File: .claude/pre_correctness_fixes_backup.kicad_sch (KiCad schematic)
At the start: 64 parts, among them J1 USB_C_Receptacle_USB2.0_16P, J10 5055670271, J12 5054482071, J2 5055670271, J3 SM04B-GHS-TB, J4 XT30 (right-angle), J5 SM04B-GHS-TB, J6 5055670271, J7 5055670271, J8 5055670271, Q1 DMP3098L-7, SW1 B3U-1000P, SW2 B3U-1000P, U1 USBLC6-2SC6, U2 AMS1117-3.3, U3 ESP32-S3-WROOM-1, U4 TJA1051T/3, U5 AP3602A, U6 LMR33630

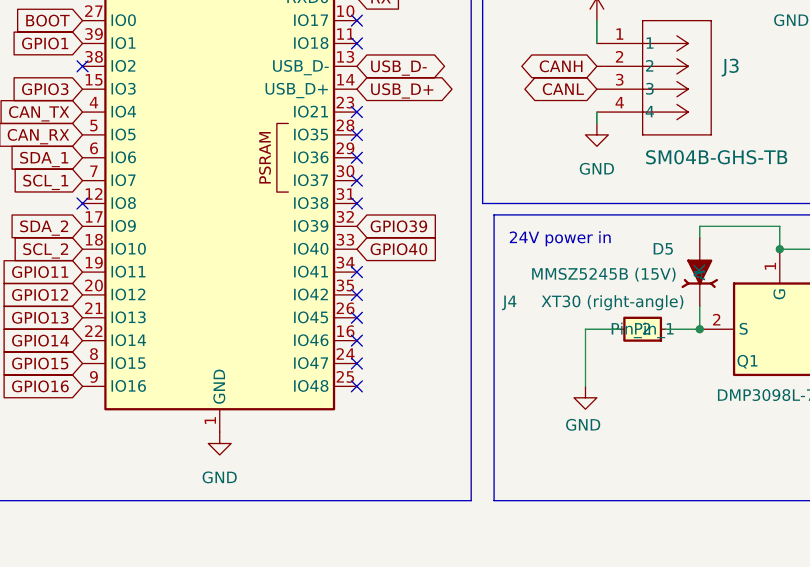
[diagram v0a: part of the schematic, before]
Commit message: Updated ready for review schematic
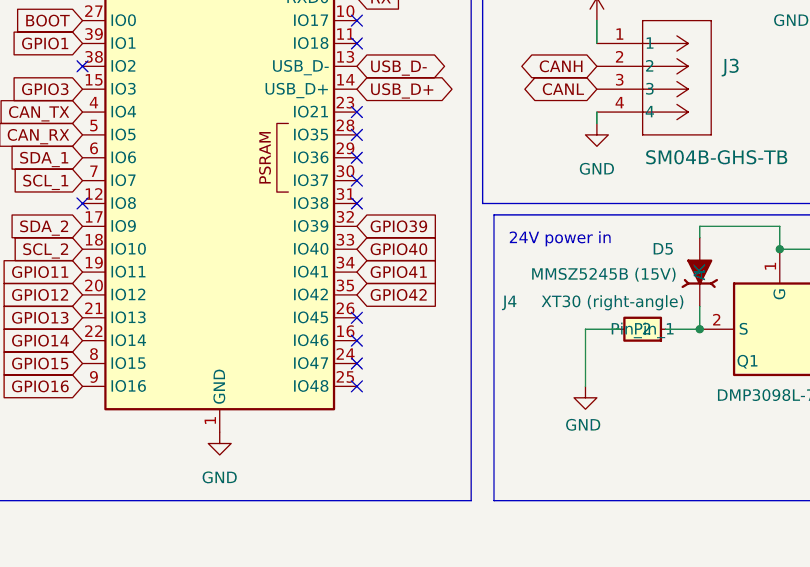
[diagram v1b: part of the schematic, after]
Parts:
- L1: footprint Footprints:L_Wurth_WE-PD-1260 -> Inductor_SMD:L_Sunlord_MWSA0603
- U6: footprint Footprints:DDA0008J -> Package_SO:HSOP-8_3.9x4.9mm_P1.27mm
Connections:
- net GPIO41: now reaches U3.34 (IO41)
- net GPIO42: now reaches U3.35 (IO42)
- no-connect marks 17 -> 15
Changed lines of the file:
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@@
 	)
 	(no_connect
-		(at 196.85 119.38)
-	)
-	(no_connect
 		(at 45.72 59.69)
 	)
@@
 	)
 	(no_connect
-		(at 196.85 121.92)
-	)
-	(no_connect
 		(at 196.85 101.6)
 	)
@@
 		)
 	)
+	(global_label "GPIO41"
+		(shape input)
+		(at 196.85 119.38 0)
+		(fields_autoplaced yes)
+		(effects
+			(font
+				(size 1.27 1.27)
+			)
+			(justify left)
+		)
+		(property "Intersheetrefs" "${INTERSHEET_REFS}"
+			(at 206.7295 119.38 0)
+			(effects
+				(font
+					(size 1.27 1.27)
+				)
+				(justify left)
+				(hide yes)
+			)
+		)
+	)
 	(global_label "GPIO3"
 		(shape input)
@@
 		)
 	)
+	(global_label "GPIO42"
+		(shape input)
+		(at 196.85 121.92 0)
+		(fields_autoplaced yes)
+		(effects
+			(font
+				(size 1.27 1.27)
+			)
+			(justify left)
+		)
+		(property "Intersheetrefs" "${INTERSHEET_REFS}"
+			(at 206.7295 121.92 0)
+			(effects
+				(font
+					(size 1.27 1.27)
+				)
+				(justify left)
+				(hide yes)
+			)
+		)
+	)
 	(global_label "SDA_2"
 		(shape input)
@@
 			)
 		)
-		(property "Footprint" "Footprints:DDA0008J"
+		(property "Footprint" "Package_SO:HSOP-8_3.9x4.9mm_P1.27mm"
 			(at 83.82 177.8 0)
 			(effects
@@
 			)
 		)
-		(property "Footprint" "Footprints:L_Wurth_WE-PD-1260"
+		(property "Footprint" "Inductor_SMD:L_Sunlord_MWSA0603"
 			(at 106.68 170.18 0)
 			(effects
@@
 	)
 	(symbol
-		(lib_id "2026-07-21_10-18-21:5055670271")
-		(at 25.4 85.09 0)
-		(unit 1)
-		(exclude_from_sim no)
-		(in_bom yes)
-		(on_board yes)
-		(dnp no)
-		(fields_autoplaced yes)
-		(property "Reference" "J2"
-			(at 39.37 85.0899 0)
-			(effects
-				(font
-					(size 1.524 1.524)
-				)
-				(justify left)
-			)
-		)
-		(property "Value" "5055670271"
-			(at 39.37 87.6299 0)
-			(effects
-				(font
-					(size 1.524 1.524)
-				)
-				(justify left)
-			)
-		)
-		(property "Footprint" "CONN_505567_02_MOL"
-			(at 25.4 85.09 0)
-			(effects
-				(font
-					(size 1.27 1.27)
-					(italic yes)
-				)
-				(hide yes)
-			)
-		)
-		(property "Datasheet" "https://www.molex.com/en-us/products/part-detail-pdf/5055670271?display=pdf"
-			(at 25.4 85.09 0)
-			(effects
-				(font
-					(size 1.27 1.27)
-					(italic yes)
-				)
-				(hide yes)
-			)
-		)
-		(property "Description" ""
-			(at 25.4 85.09 0)
-			(effects
-				(font
-					(size 1.27 1.27)
-				)
-				(hide yes)
-			)
-		)
-		(pin "2"
-		)
-		(pin "1"
-		)
-		(instances
-			(project "First_ESP32"
-				(path "/cb438fcd-98ad-4b96-995d-9cc141a4f6d9/2e9f25ce-3924-4476-88a9-39de14992abb"
-					(reference "J2")
-					(unit 1)
-				)
-			)
-		)
-	)
-	(symbol
 		(lib_id "Device:C")
 		(at 255.27 54.61 0)
@@
 					(unit 1)
 				)
+			)
+		)
+	)
+	(symbol
+		(lib_id "2026-07-21_10-18-21:5055670271")
+		(at 25.4 85.09 0)
+		(unit 1)
+		(exclude_from_sim no)
+		(in_bom yes)
+		(on_board yes)
+		(dnp no)
+		(fields_autoplaced yes)
+		(property "Reference" "J2"
+			(at 39.37 85.0899 0)
+			(effects
+				(font
+					(size 1.524 1.524)
+				)
+				(justify left)
+			)
+		)
+		(property "Value" "5055670271"
+			(at 39.37 87.6299 0)
+			(effects
+				(font
+					(size 1.524 1.524)
+				)
+				(justify left)
+			)
+		)
+		(property "Footprint" "CONN_505567_02_MOL"
+			(at 25.4 85.09 0)
+			(effects
+				(font
+					(size 1.27 1.27)
+					(italic yes)
+				)
+				(hide yes)
+			)
+		)
+		(property "Datasheet" "https://www.molex.com/en-us/products/part-detail-pdf/5055670271?display=pdf"
+			(at 25.4 85.09 0)
+			(effects
+				(font
+					(size 1.27 1.27)
+					(italic yes)
+				)
+				(hide yes)
+			)
+		)
+		(property "Description" ""
+			(at 25.4 85.09 0)
+			(effects
+				(font
+					(size 1.27 1.27)
+				)
+				(hide yes)
+			)
+		)
+		(pin "2"
+		)
+		(pin "1"
+		)
+		(instances
+			(project "First_ESP32"
+				(path "/cb438fcd-98ad-4b96-995d-9cc141a4f6d9/2e9f25ce-3924-4476-88a9-39de14992abb"
+					(reference "J2")
+					(unit 1)
+				)
